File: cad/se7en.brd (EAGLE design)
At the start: 64.1 x 34 mm, 59 parts, among them CN1 MICROSD-EJECT, CN3 DO NOT PLACE, CN4 DO NOT PLACE, SW1 SWITCHKMR211, SW2 SWITCHKMR211, U1 ATSAME70, X1 12MHz, X2 32k768

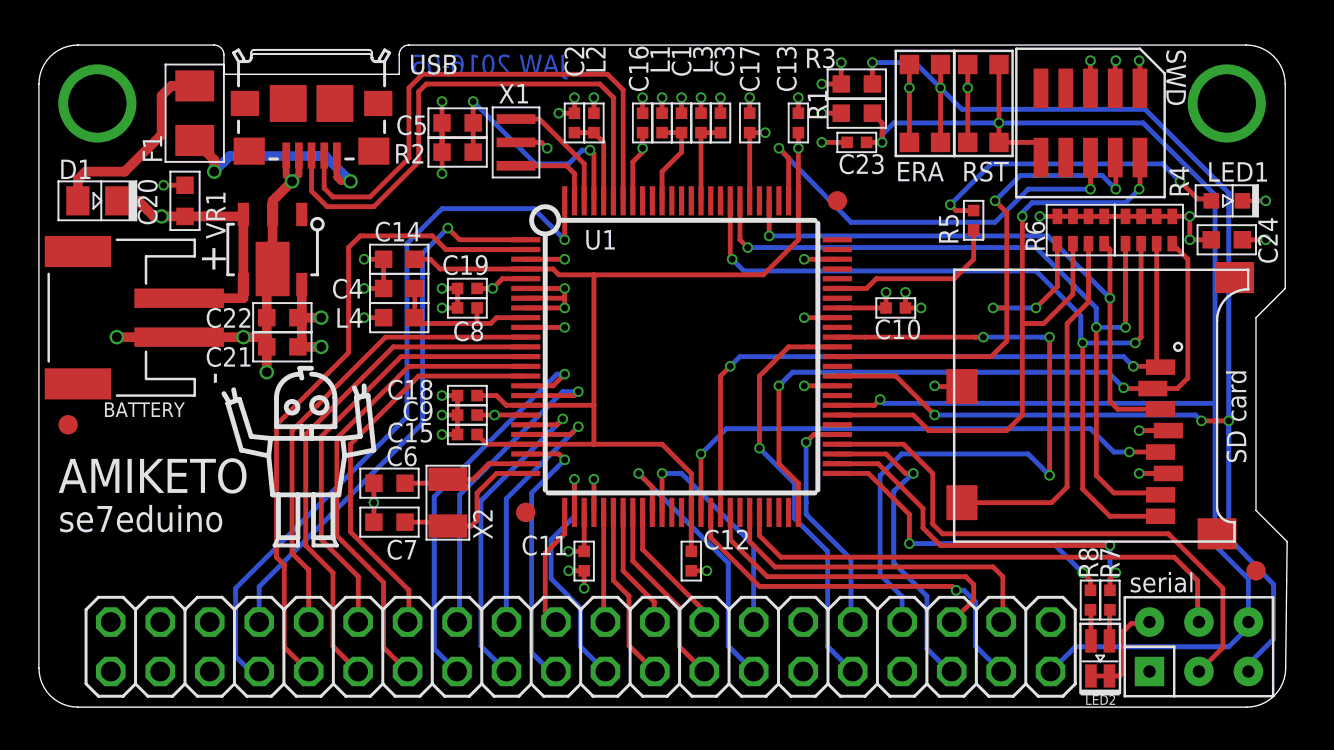
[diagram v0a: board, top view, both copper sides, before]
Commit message: charger
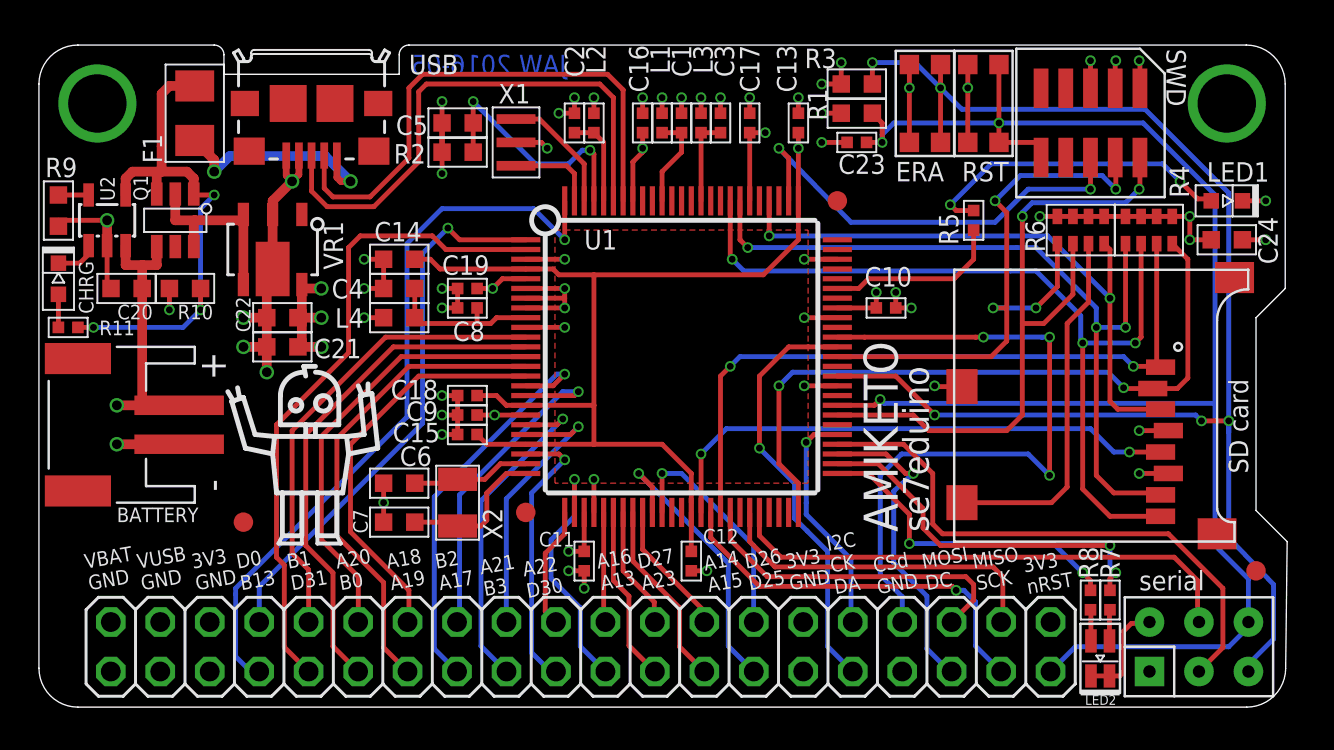
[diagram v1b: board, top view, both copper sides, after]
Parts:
- removed D1: 1A, jaw:SMD0805D
- added LED3: LED, jaw:SMD0603D
- added Q1: FDC6329S, jaw:SOT-23-6
- added R10: 1M, jaw:SMD0603
- added R11: 1k, jaw:SMD0402
- added R9: 10k, jaw:SMD0603
- added U2: MCP73831/OT, adafruit:SOT23-5L
- C1: value 4u7 -> .1u
- C2, C3: value (none) -> .1u
- L1: value 10u -> 1u
- L2, L3: value (none) -> 1u
- moved U$4 10.3 mm to (66.5, 44.5)
- moved CN2 5.50 mm to (59.5, 49.5)
- moved C20 5.41 mm to (60.5, 56.5), turned to 180 degrees
- moved C10 0.50 mm to (99.5, 55.5)
- moved C6 0.50 mm to (74.5, 46.5)
- moved C7 0.50 mm to (74.5, 44.5)
- moved X2 0.50 mm to (77.5, 45.5)
- moved U$3 0.22 mm to (69.9, 47.8)
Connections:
- removed net N$15: D1.A, F1.2
- new net N$10: LED3.C, U2.1
- new net N$12: LED3.A, R11.1
- new net N$17: R9.1, U2.5
- new net VIN: F1.2, Q1.1, Q1.3, R10.2, R11.2, U2.4
- new net VSYS: Q1.2, Q1.6, VR1.3, VR1.4
- net GND: now also R10.1, R9.2, U2.2
- net VBAT: now also Q1.4, U2.3; no longer D1.C, VR1.3, VR1.4
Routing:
- net VIN: track 0.00 -> 27.5 mm, vias 0 -> 3
- net N$15: track 10.3 -> 0.00 mm
- net VSYS: track 0.00 -> 9.82 mm
- net VBAT: track 41.5 -> 32.7 mm
- net GND: track 89.0 -> 94.3 mm, vias 46 -> 48
- net N$10: track 0.00 -> 2.19 mm
- net N$12: track 0.00 -> 1.70 mm
- net N$17: track 0.00 -> 1.55 mm
- net N$9: track 8.22 -> 7.67 mm
- net N$11: track 6.61 -> 6.06 mm
- net VCC: track 44.8 -> 45.3 mm, vias 17 -> 18
- added copper zone on layer 1, net V1V2
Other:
- board text added: "3V3 GND"
- board text added: "3V3 nRST"
- board text added: "A14 A15"
- board text added: "A16 A13"
- board text added: "A18 A19"
- board text added: "A20 B0"
- board text added: "A21 B3"
- board text added: "A22 D30"
- board text added: "B1 D31"
- board text added: "B2 A17"
- board text added: "CHRG"
- board text added: "CSd GND"
- board text added: "D0 B13"
- board text added: "D26 D25"
- board text added: "D27 A23"
- board text added: "I2C CK DA"
- board text added: "MISO SCK"
- board text added: "MOSI DC"
- board text added: "VBAT GND"
- board text added: "VUSB GND"

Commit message: tweak
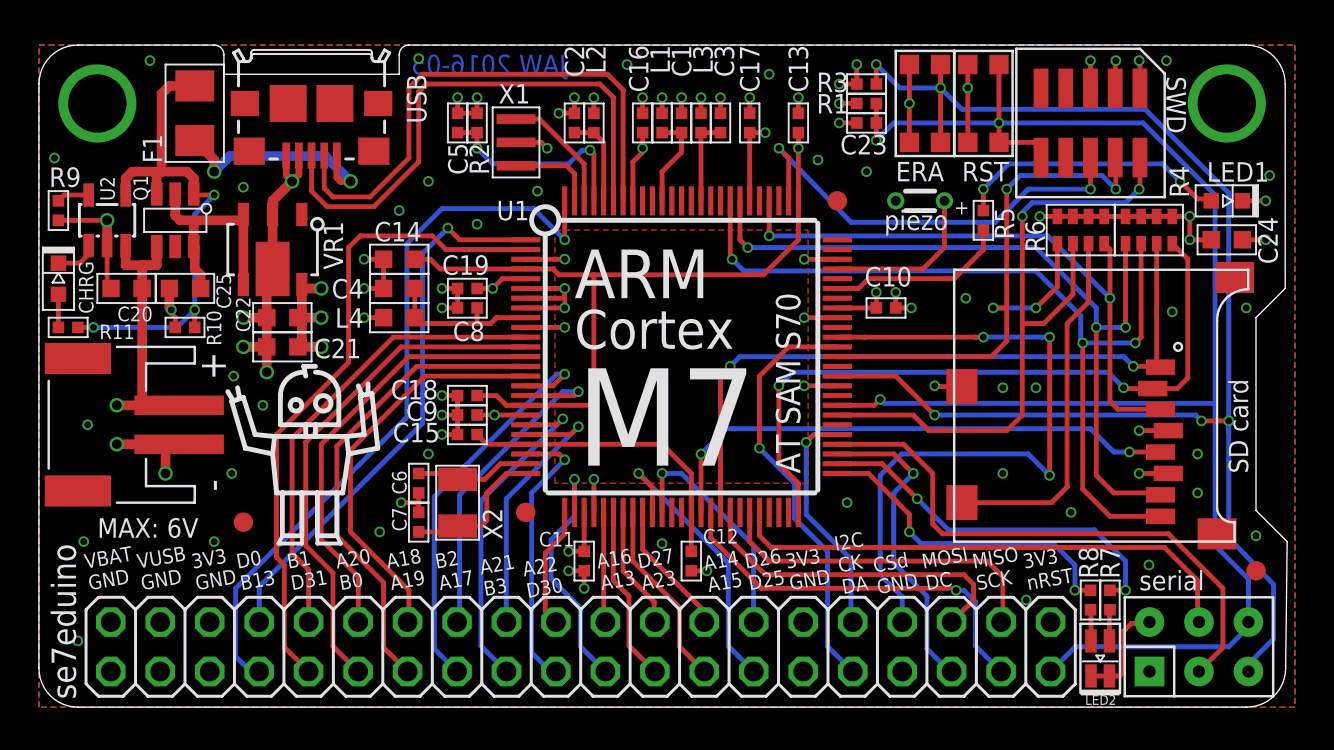
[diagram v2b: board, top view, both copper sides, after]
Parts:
- added C25: 10u, jaw:SMD0603
- added CN6, CN7: DO NOT PLACE, jaw:HEADER-1X1-SMALL
- C5, C6, C7, R1, R10, R2, R3, R9: device jaw:SMD0603 -> jaw:SMD0402
- CN5: value (none) -> DO NOT PLACE
- L1, L2, L3: value 1u -> FB
- LED1: value LED -> white
- LED3: value LED -> RED
- moved U$1 31.1 mm to (91.2, 58.4)
- moved LOGO1 30.4 mm to (97.9, 55.7)
- moved R10 2.00 mm to (63.5, 54.5)
- moved R2 1.80 mm to (78.5, 65.0), turned to 270 degrees
- moved C23 1.12 mm to (98.5, 65.0)
- moved C6 1.00 mm to (75.5, 46.5), turned to 270 degrees
- moved C7 1.00 mm to (75.5, 44.5), turned to 90 degrees
- moved R1 0.71 mm to (98.5, 66.0)
- moved R3 0.50 mm to (98.5, 67.0)
- moved R5 0.50 mm to (104.5, 60.0)
- turned C5 to 90 degrees
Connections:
- new net PIEZO: CN7.P$1, U1.72
- new net PINA12: U1.48
- net GND: now also C25.2, CN6.P$1
- net VSYS: now also C25.1
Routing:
- net PIEZO: track 0.00 -> 8.36 mm
- net N$16: track 16.4 -> 14.1 mm
- net VSYS: track 9.82 -> 12.0 mm
- net N$7: track 12.9 -> 10.9 mm
- net GND: track 94.3 -> 93.3 mm, vias 48 -> 86
- net NRST: track 82.4 -> 81.8 mm
- added copper zone on layer 1, net GND
- added copper zone on layer 16, net GND
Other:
- board text added: "+"
- board text added: "34mm"
- board text added: "64mm"
- board text added: "ARM"
- board text added: "AT SAM S70"
- board text added: "Cortex"
- board text added: "M7"
- board text added: "MAX: 6V"
- board text added: "Pb"
- board text added: "piezo"
- board text removed: "AMIKETO"
- board text removed: "BATTERY"
